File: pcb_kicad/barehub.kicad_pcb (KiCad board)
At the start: 2 copper layers, 51.4 x 96.2 mm, 36 parts, among them J2 USB_A, J3 USB_A, J4 USB_A, J5 USB_A, J6 USB_C_Receptacle_USB2.0_16P, U1 FE1.1s, U2 SMF05CT1G, U3 SMF05CT1G, U4 SMF05CT1G, U5 SMF05CT1G, U6 SMF05CT1G, Y1 12Mhz

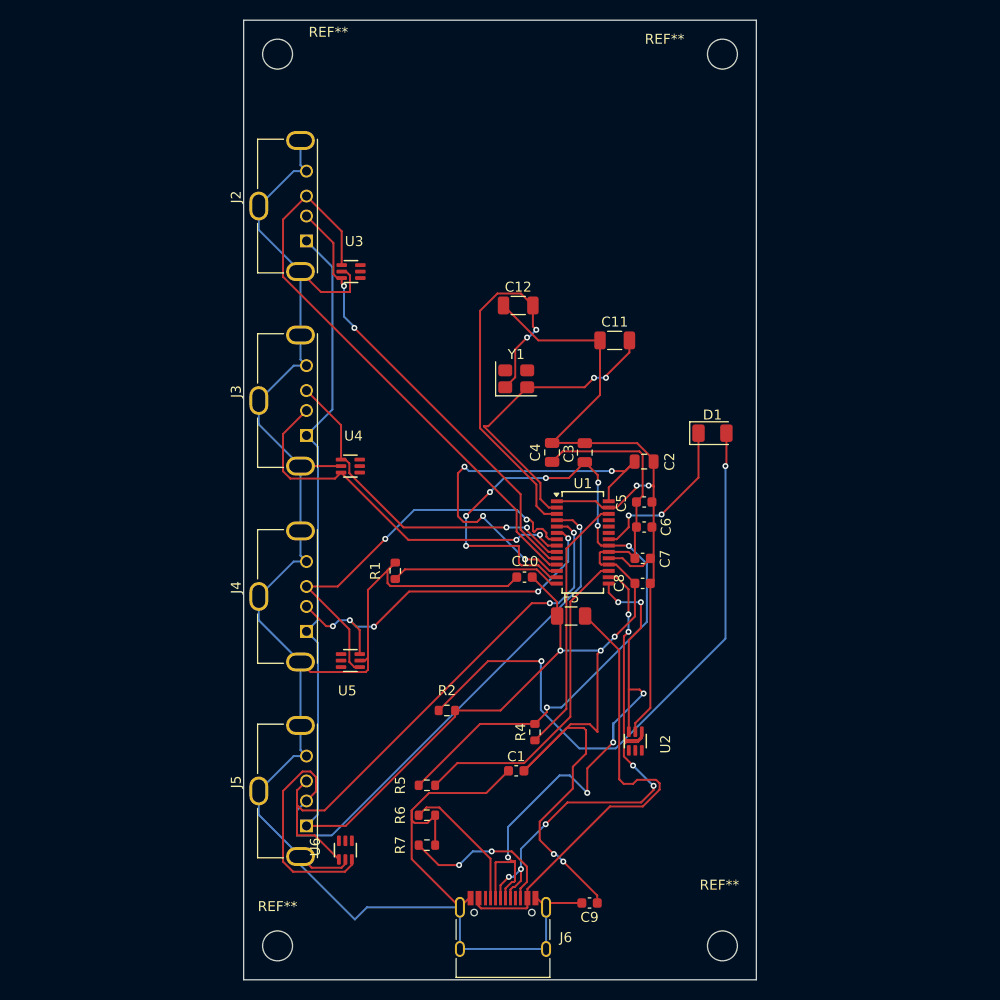
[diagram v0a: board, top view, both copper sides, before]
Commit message: chore: add BOM
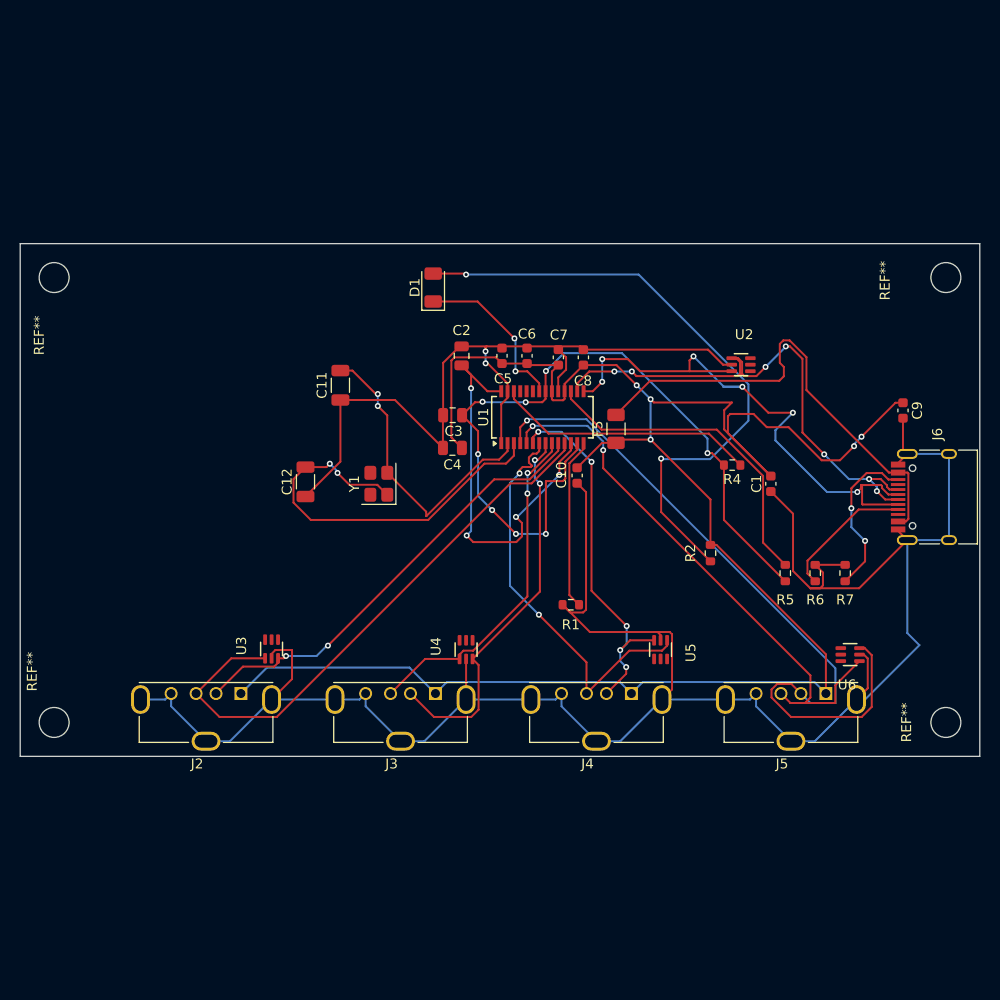
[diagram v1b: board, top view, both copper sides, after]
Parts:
- moved REF** 70.6 mm to (100.8, 57.6), turned to 90 degrees
- moved REF** 70.6 mm to (190.2, 57.6), turned to 90 degrees
- moved REF** 70.6 mm to (100.8, 102.2), turned to 90 degrees
- moved REF** 70.6 mm to (190.2, 102.2), turned to 90 degrees
- moved J6 62.2 mm to (189.5, 79.6), turned to 90 degrees
- moved C9 58.5 mm to (185.9, 70.9), turned to -90 degrees
- moved U6 54.3 mm to (180.6, 95.4), turned to 180 degrees
- moved J5 53.7 mm to (178.2, 99.3), turned to 180 degrees
- moved R7 50.0 mm to (180.1, 87.2), turned to 90 degrees
- moved R6 45.9 mm to (177.1, 87.2), turned to 90 degrees
- moved J2 45.8 mm to (119.5, 99.3), turned to 180 degrees
- moved R5 41.8 mm to (174.1, 87.2), turned to 90 degrees
- moved U2 39.2 mm to (169.7, 66.3), turned to 0 degrees
- moved U3 38.7 mm to (122.6, 94.8), turned to 90 degrees
- moved C1 38.5 mm to (172.7, 78.3), turned to 90 degrees
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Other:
- board size 51.4 x 96.2 mm -> 96.2 x 51.4 mm
